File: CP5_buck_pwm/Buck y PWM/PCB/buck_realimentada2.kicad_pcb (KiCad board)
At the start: 2 copper layers, 95 x 89 mm, 42 parts, among them J1 Vin, J2 Vout, M3 IRFZ44N, M4 IRFZ44N, U1 IR2104, U2 LM393, U3 TL084, U4 LM317_TO-220, U5 TL431LP

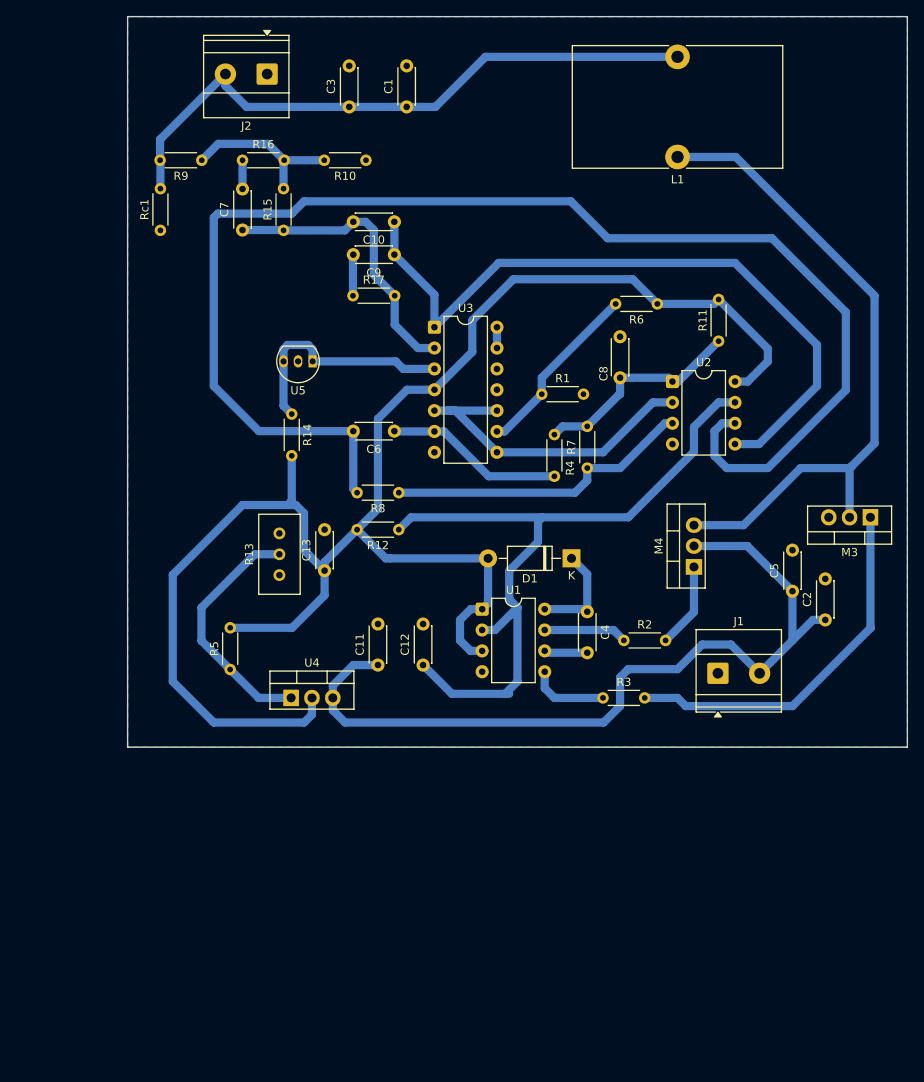
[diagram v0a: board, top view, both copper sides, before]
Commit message: PCB terminado
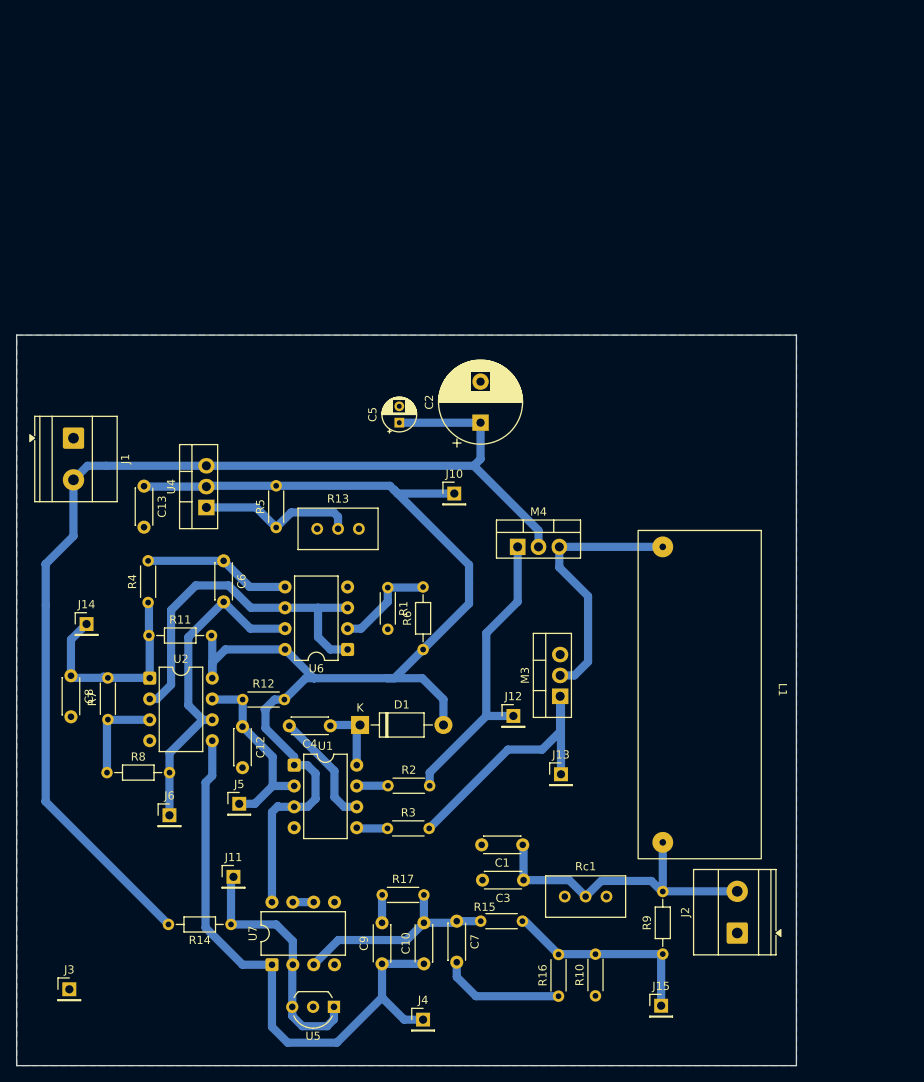
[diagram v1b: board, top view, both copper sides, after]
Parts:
- removed C11: 0.1u, Capacitor_THT:C_Disc_D4.3mm_W1.9mm_P5.00mm
- removed U3: TL084, Package_DIP:DIP-14_W7.62mm
- added J10: Conn_vcc, Connector_PinHeader_2.54mm:PinHeader_1x01_P2.54mm_Vertical, F.Cu at (151.8, 77.1)
- added J11: Conn_vref, Connector_PinHeader_2.54mm:PinHeader_1x01_P2.54mm_Vertical, F.Cu at (124.9, 123.8)
- added J12: Conn_vg1, Connector_PinHeader_2.54mm:PinHeader_1x01_P2.54mm_Vertical, F.Cu at (159.0, 104.2)
- added J13: Conn_vg2, Connector_PinHeader_2.54mm:PinHeader_1x01_P2.54mm_Vertical, F.Cu at (164.8, 111.3)
- added J14: Conn_cuadrada, Connector_PinHeader_2.54mm:PinHeader_1x01_P2.54mm_Vertical, F.Cu at (107.0, 93.0)
- added J15: Conn_sampling, Connector_PinHeader_2.54mm:PinHeader_1x01_P2.54mm_Vertical, F.Cu at (177.0, 139.5)
- added J3: Conn_gnd, Connector_PinHeader_2.54mm:PinHeader_1x01_P2.54mm_Vertical, F.Cu at (104.9, 137.5)
- added J4: Conn_error, Connector_PinHeader_2.54mm:PinHeader_1x01_P2.54mm_Vertical, F.Cu at (148.0, 141.2)
- added J5: Conn_pwm, Connector_PinHeader_2.54mm:PinHeader_1x01_P2.54mm_Vertical, F.Cu at (125.6, 114.9)
- added J6: Conn_triangular, Connector_PinHeader_2.54mm:PinHeader_1x01_P2.54mm_Vertical, F.Cu at (117.1, 116.3)
- added U6: TL082, Package_DIP:DIP-8_W7.62mm, F.Cu at (138.8, 96.1)
- added U7: TL082, Package_DIP:DIP-8_W7.62mm, F.Cu at (129.6, 134.5)
- C2: footprint Capacitor_THT:C_Disc_D4.3mm_W1.9mm_P5.00mm -> Capacitor_THT:CP_Radial_D10.0mm_P5.00mm
- C5: footprint Capacitor_THT:C_Disc_D4.3mm_W1.9mm_P5.00mm -> Capacitor_THT:CP_Radial_D4.0mm_P2.00mm
- L1: footprint Inductor_THT:L_Toroid_Vertical_L25.4mm_W14.7mm_P12.20mm_Vishay_TJ5_BigPads -> inductor:Untitled
- R11, R14, R6, R8, R9: footprint Resistor_THT:R_Axial_DIN0204_L3.6mm_D1.6mm_P5.08mm_Horizontal -> Resistor_THT:R_Axial_DIN0204_L3.6mm_D1.6mm_P7.62mm_Horizontal
- Rc1: footprint Resistor_THT:R_Axial_DIN0204_L3.6mm_D1.6mm_P5.08mm_Horizontal -> Potentiometer_THT:Potentiometer_Bourns_3296W_Vertical
- U5: footprint Package_TO_SOT_THT:TO-92_Inline -> Package_TO_SOT_THT:TO-92_Inline_Wide
- moved J2 119.3 mm to (186.3, 130.6), turned to 90 degrees
- moved R9 111.8 mm to (177.2, 133.2), turned to 90 degrees
- moved R16 108.9 mm to (164.5, 138.3), turned to 90 degrees
- moved R10 105.6 mm to (169.0, 138.3), turned to 90 degrees
- moved Rc1 97.7 mm to (170.3, 126.2), turned to 0 degrees
- moved C3 96.6 mm to (160.2, 124.2), turned to 180 degrees
- moved C1 91.0 mm to (160.1, 119.9), turned to 180 degrees
- moved C10 90.5 mm to (148.1, 134.4), turned to 90 degrees
- moved C7 88.2 mm to (152.1, 129.2), turned to -90 degrees
- moved R15 87.5 mm to (155.0, 129.2), turned to 0 degrees
- moved C9 86.4 mm to (143.0, 134.4), turned to 90 degrees
- moved J1 83.6 mm to (105.4, 70.4), turned to -90 degrees
- moved U5 78.7 mm to (137.1, 139.6)
- moved R11 78.1 mm to (114.6, 94.4), turned to 0 degrees
- moved C8 76.1 mm to (105.1, 99.3), turned to -90 degrees
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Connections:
- R14 pad 2: VCCPWM -> Vin
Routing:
- net Triangular: track 166.8 -> 40.4 mm
- net pwm: track 90.7 -> 24.1 mm
- net VCCPWM: track 206.1 -> 150.6 mm
- net Vd: track 81.5 -> 32.1 mm
- net Vin: track 100.6 -> 139.9 mm
- net Vout: track 77.4 -> 38.5 mm
- net Vg1: track 10.4 -> 36.8 mm
- net Net-(U2A-+): track 37.7 -> 11.6 mm
- net error: track 86.8 -> 72.5 mm
- net Net-(C7-Pad2): track 3.50 -> 15.2 mm
- net Net-(U4-ADJ): track 30.0 -> 19.5 mm
- net Vg2: track 45.4 -> 35.0 mm
- net Net-(U6A--): track 22.1 -> 12.3 mm
- net Net-(U7A-+): track 35.5 -> 25.9 mm
- net Net-(U1-VS): track 5.28 -> 14.2 mm
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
